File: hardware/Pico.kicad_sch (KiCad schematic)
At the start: 36 parts, among them J1 Conn_01x03 2.54mm, J5 Conn_01x04, J6 Conn_01x06, J7 Conn_01x12, U10 SRV05-4, U6 SRV05-4, U7 SRV05-4, U9 SRV05-4

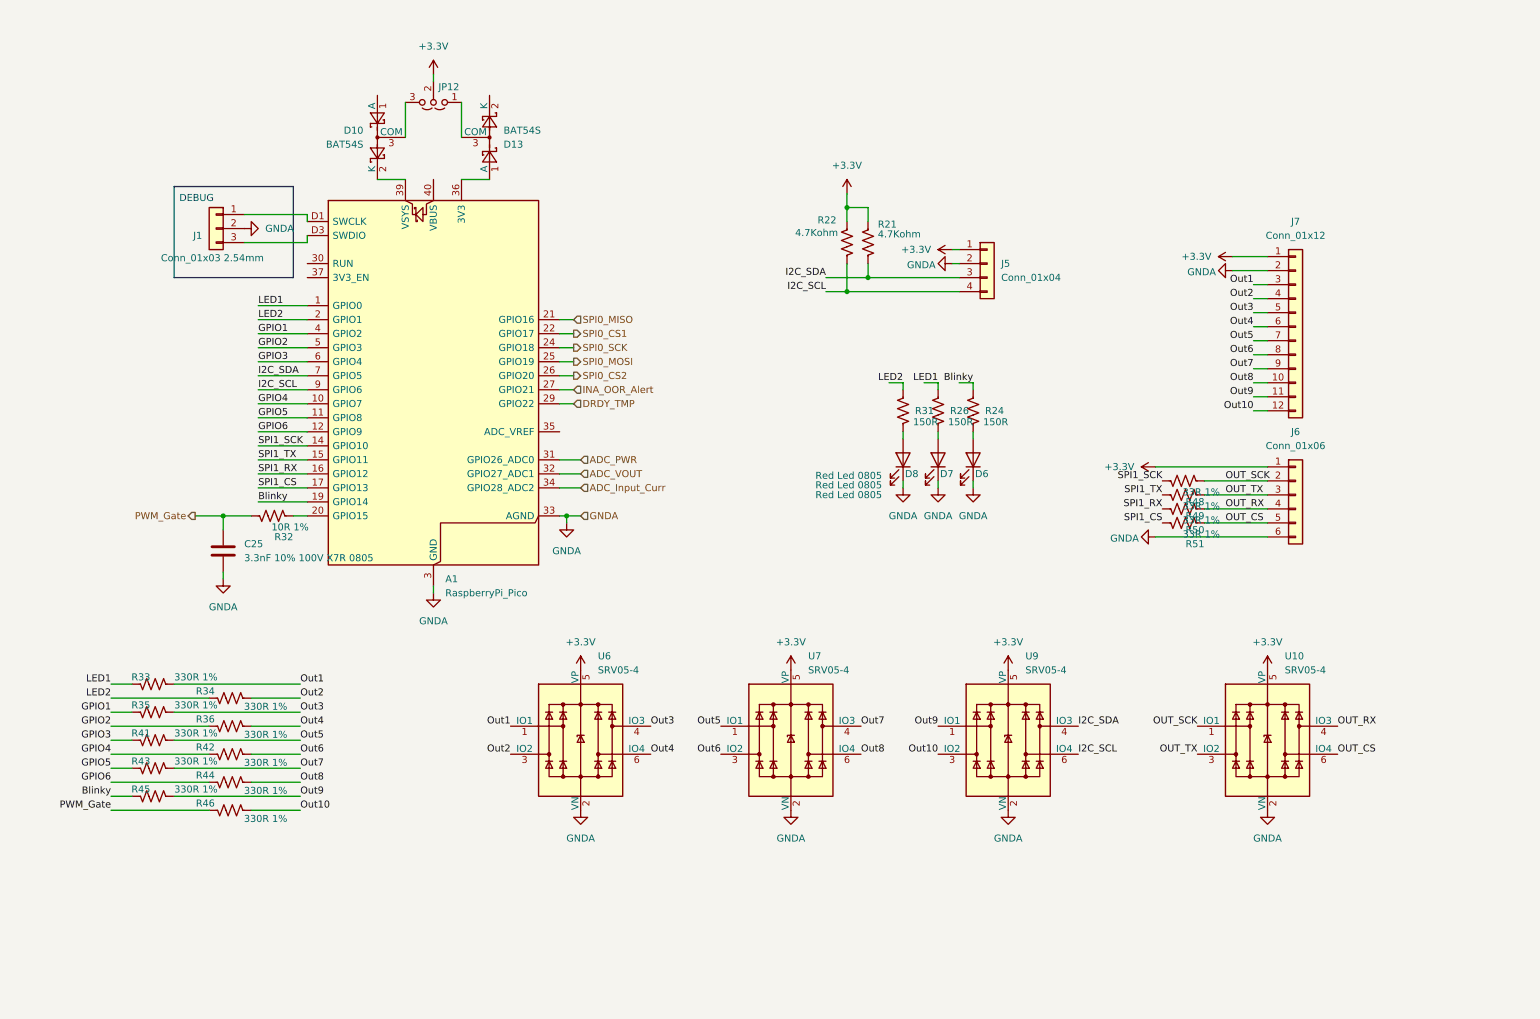
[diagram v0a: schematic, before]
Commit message: HW: Changes in GPIO components. PCB WIP
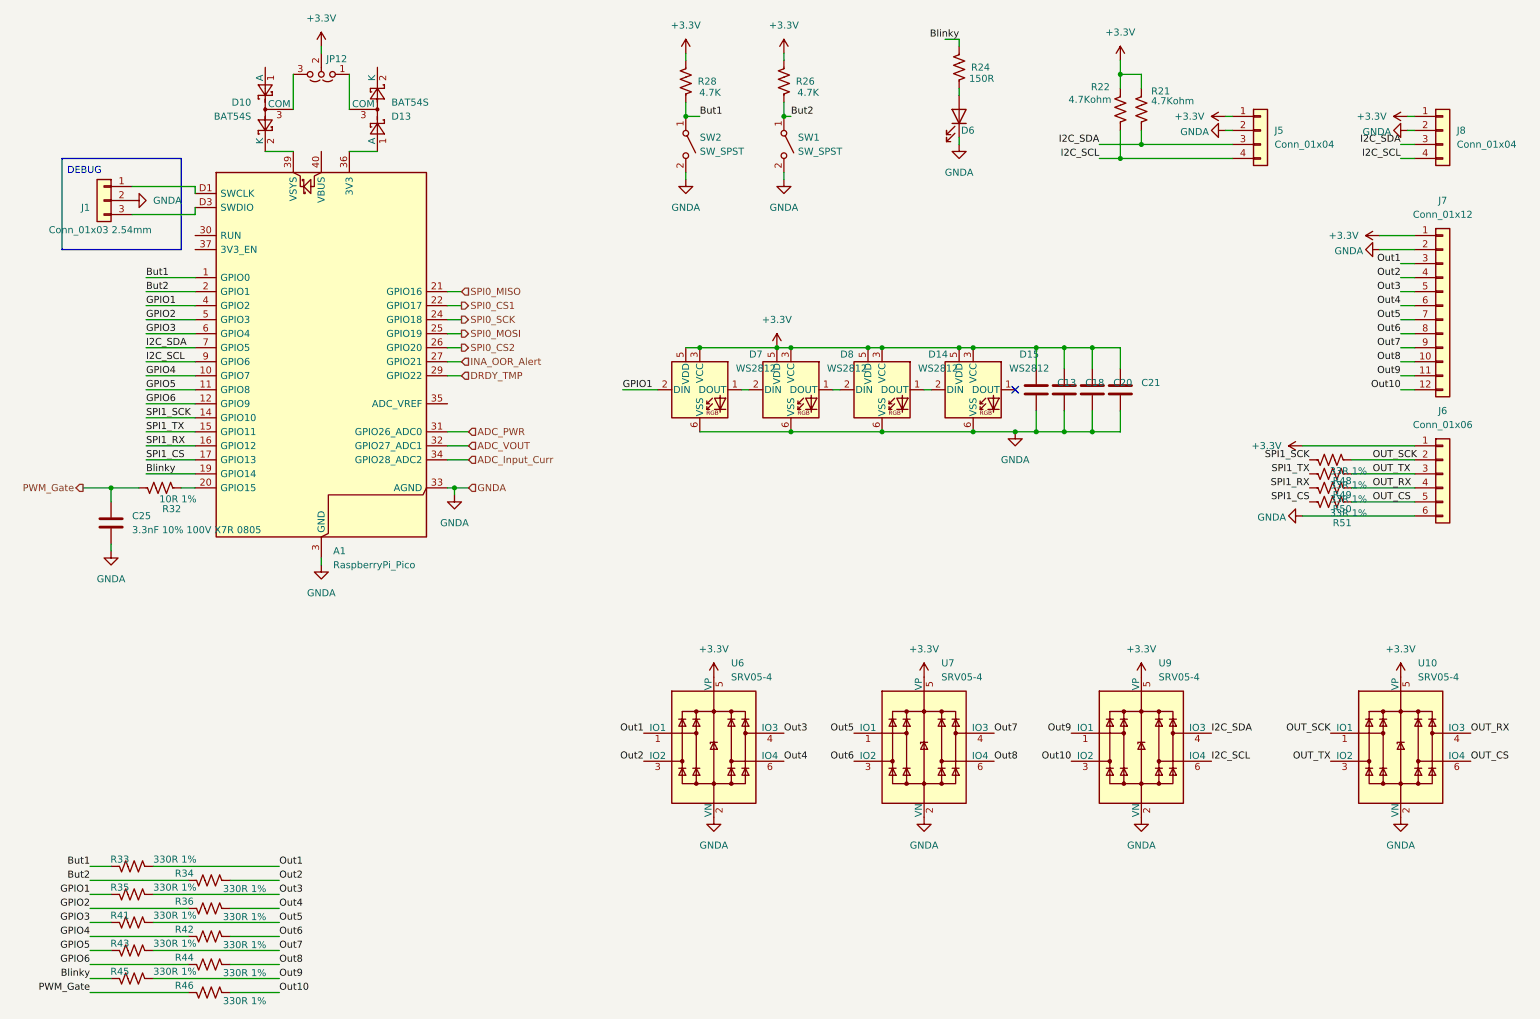
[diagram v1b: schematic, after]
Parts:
- removed D7, D8: Red Led 0805, LED_SMD:LED_0805_2012Metric_Pad1.15x1.40mm_HandSolder, symbol Device:LED
- removed R31: 150R, Resistor_SMD:R_0805_2012Metric_Pad1.20x1.40mm_HandSolder, symbol Device:R_US
- added C13, C18, C20, C21: 100nF 10% 100V X7R 0805, Capacitor_SMD:C_0805_2012Metric_Pad1.18x1.45mm_HandSolder, symbol Device:C
- added D14, D15, D7, D8: WS2812, LED_SMD:LED_WS2812_PLCC6_5.0x5.0mm_P1.6mm, symbol LED:WS2812
- added J8: Conn_01x04, Connector_PinHeader_2.54mm:PinHeader_1x04_P2.54mm_Vertical, symbol Connector_Generic:Conn_01x04
- added R28: 4.7K, Resistor_SMD:R_0805_2012Metric_Pad1.20x1.40mm_HandSolder, symbol Device:R_US
- added SW1, SW2: SW_SPST, Button_Switch_SMD:SW_Push_1TS009xxxx-xxxx-xxxx_6x6x5mm, symbol Switch:SW_SPST
- R26: value 150R -> 4.7K; LCSC Part C153298 -> (none)
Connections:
- net LED2 is gone; now on net But2: A1.2 (GPIO1), R34.1
- net +3.3V: now also R26.1, C13.1, C18.1, C20.1, C21.1, D14.3 (VCC), D14.5 (VDD), D15.3 (VCC), D15.5 (VDD), D7.3 (VCC), D7.5 (VDD), D8.3 (VCC), D8.5 (VDD), J8.1 (Pin_1), R28.1
- net GNDA: now also C13.2, C18.2, C20.2, C21.2, D14.6 (VSS), D15.6 (VSS), D7.6 (VSS), D8.6 (VSS), J8.2 (Pin_2), SW1.2 (B), SW2.2 (B)
- net GPIO1: now also D7.2 (DIN)
- net I2C_SCL: now also J8.4 (Pin_4)
- net I2C_SDA: now also J8.3 (Pin_3)
- net But2: now reaches R26.2
- net But2: now also SW1.1 (A)
- net LED1 renamed But1
- net But1: now also R28.2, SW2.1 (A); no longer R26.1
- new net: D14.1 (DOUT), D15.2 (DIN)
- new net: D7.1 (DOUT), D8.2 (DIN)
- new net: D14.2 (DIN), D8.1 (DOUT)
- no-connect marks 0 -> 1
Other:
- moved on the sheet: A1, C25, D10, D13, D6, J1, J5, J6, J7, JP12, R21, R22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
